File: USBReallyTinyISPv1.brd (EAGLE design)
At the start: 26 x 16.5 mm, 20 parts, among them IC1 ATTINY2313, IC2 74AC125D, Q1 12 MHz, X1 miniUSB-B

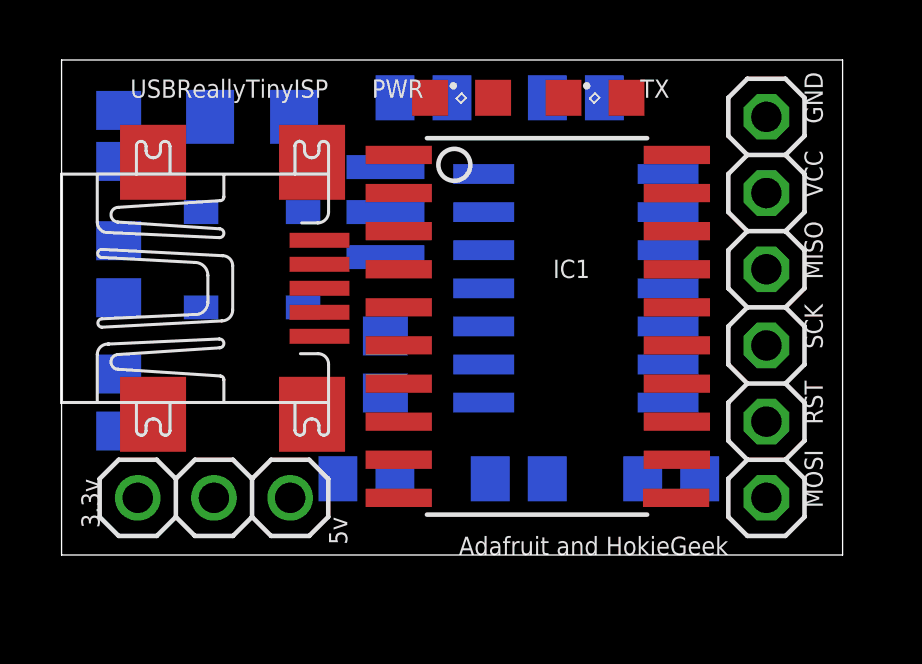
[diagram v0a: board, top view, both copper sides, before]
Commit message: Lots of tweaks to get a tiny little board!
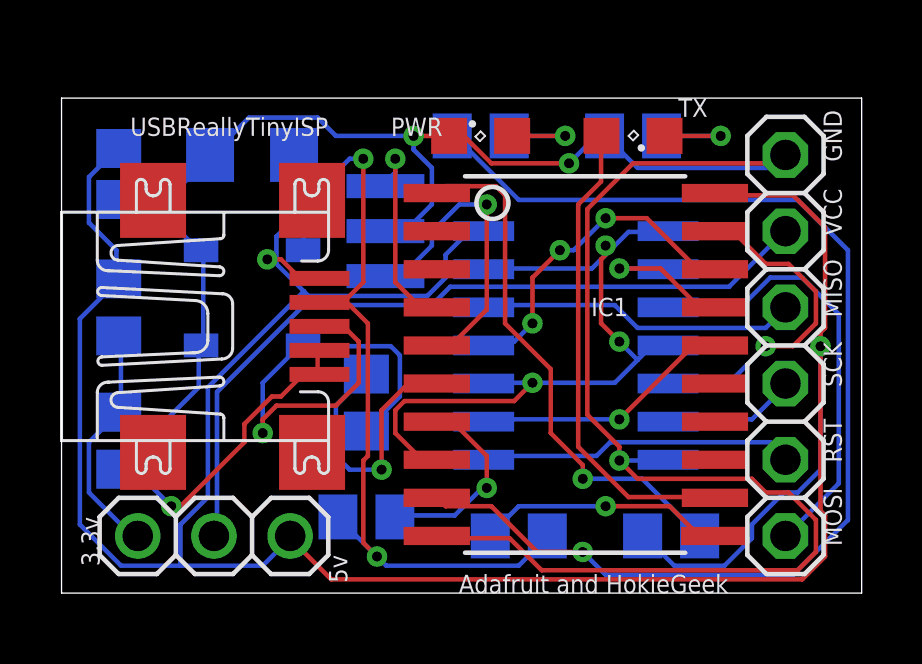
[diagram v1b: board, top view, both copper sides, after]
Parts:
- moved R1 2.29 mm to (19.1, 15.2), turned to 180 degrees
- moved R2 2.29 mm to (14.0, 15.2)
- moved R5 1.91 mm to (15.2, 1.91)
- moved R6 1.91 mm to (20.3, 1.91)
- moved IC2 1.90 mm to (17.1, 8.26)
- moved LED1 1.80 mm to (19.1, 15.2), turned to 180 degrees
- moved IC1 1.80 mm to (17.1, 7.62)
- moved LED2 1.42 mm to (14.0, 15.2)
- moved R3 1.42 mm to (10.2, 6.35)
- moved JP2 1.42 mm to (24.1, 8.26)
- moved R4 1.27 mm to (10.2, 2.54)
- moved JP1 1.27 mm to (5.08, 1.91)
- moved C1 1.27 mm to (1.91, 14.0)
- moved C2 1.27 mm to (6.35, 14.6)
- moved D1 1.27 mm to (6.35, 11.4)
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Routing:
- net VCC: track 0.00 -> 93.8 mm, vias 0 -> 2
- net GND: track 0.00 -> 90.6 mm, vias 0 -> 4
- net N$5: track 0.00 -> 39.3 mm, vias 0 -> 1
- net N$11: track 0.00 -> 28.0 mm, vias 0 -> 2
- net N$13: track 0.00 -> 26.0 mm
- net N$12: track 0.00 -> 25.4 mm, vias 0 -> 3
- net N$4: track 0.00 -> 17.7 mm, vias 0 -> 1
- net N$10: track 0.00 -> 16.9 mm, vias 0 -> 1
- net N$1: track 0.00 -> 16.0 mm
- net MOSI: track 0.00 -> 14.8 mm
- net MISO': track 0.00 -> 11.1 mm, vias 0 -> 3
- net SCK': track 0.00 -> 11.0 mm, vias 0 -> 1
- net MISO: track 0.00 -> 10.7 mm
- net RST: track 0.00 -> 10.6 mm
- net N$3: track 0.00 -> 10.3 mm, vias 0 -> 1
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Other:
- board size 26 x 16.5 mm -> 26.7 x 16.5 mm
- board text removed: "0.1uF"
- board text removed: "1.5k"
- board text removed: "100uF"
- board text removed: "10k"
- board text removed: "12Mhz"
- board text removed: "3.6v"
- board text removed: "47"
- board text removed: "47k"
- board text removed: "91k"
